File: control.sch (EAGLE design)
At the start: 63 parts

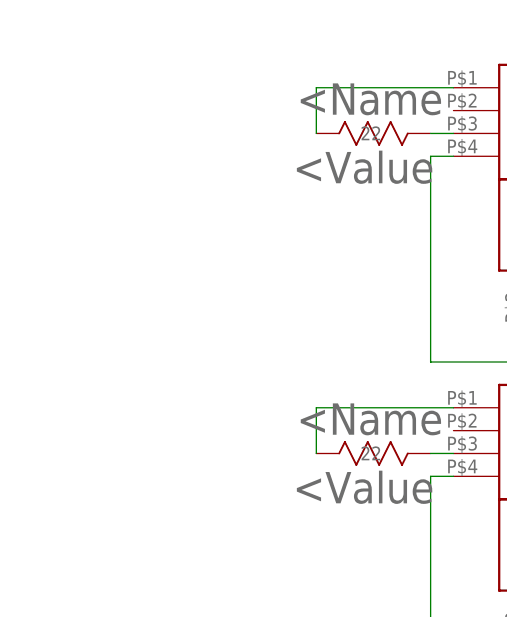
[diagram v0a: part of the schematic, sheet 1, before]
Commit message: Revert "Merge remote-tracking branch 'refs/remotes/origin/master' into new-layout"
This reverts commit d786cf153478cbc5e1d0f0cbdb23b775e7a3effd.
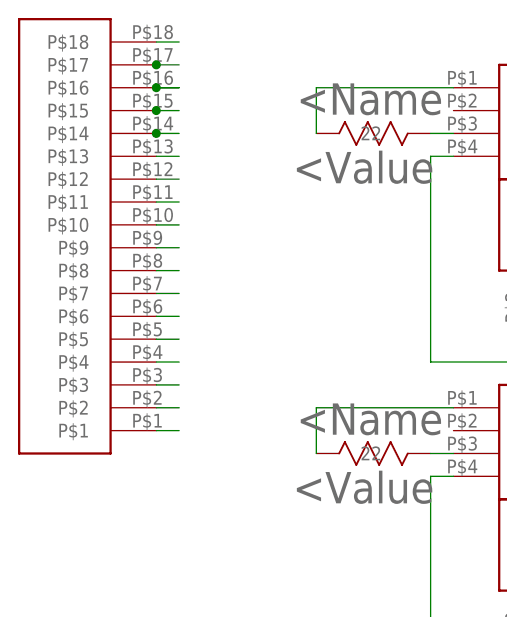
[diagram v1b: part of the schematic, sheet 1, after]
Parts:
- U$39: value MOTORCONNECTOR -> SFV18R-3STBE1HLF; device Smile_Shade:MOTORCONNECTOR -> Smile_Shade:SFV18R-3STBE1HLF
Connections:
- net LEDSTR_1: now also U$39.P$18
- net LEDSTR_10: now also U$39.P$9
- net LEDSTR_11: now also U$39.P$10
- net LEDSTR_12: now also U$39.P$7
- net LEDSTR_13: now also U$39.P$6
- net LEDSTR_14: now also U$39.P$5
- net LEDSTR_15: now also U$39.P$4
- net LEDSTR_16: now also U$39.P$3
- net LEDSTR_17: now also U$39.P$1
- net LEDSTR_18: now also U$39.P$2
- net LEDSTR_2: now also U$39.P$17
- net LEDSTR_3: now also U$39.P$16
- net LEDSTR_4: now also U$39.P$15
- net LEDSTR_5: now also U$39.P$12
- net LEDSTR_6: now also U$39.P$13
- net LEDSTR_7: now also U$39.P$14
- net LEDSTR_8: now also U$39.P$11
- net LEDSTR_9: now also U$39.P$8
- net M1A: no longer U$38.MB
- net M1B: no longer U$38.MA
- net M2A: now also U$38.MA; no longer U$39.MA
- net M2B: now also U$38.MB; no longer U$39.MB
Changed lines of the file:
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@@
 <part name="U$37" library="Smile_Shade" deviceset="PCA9685PW/Q900" device=""/>
 <part name="U$38" library="Smile_Shade" deviceset="MOTORCONNECTOR" device=""/>
-<part name="U$39" library="Smile_Shade" deviceset="MOTORCONNECTOR" device=""/>
 <part name="U$40" library="LED Driver" deviceset="NUD4011DR2G" device=""/>
 <part name="U$41" library="LED Driver" deviceset="2N7002P" device=""/>
@@
 <part name="U$43" library="LED Driver" deviceset="2N7002P" device=""/>
 <part name="R18" library="LED Driver" deviceset="RC0603FR-0710RL" device=""/>
+<part name="U$39" library="Smile_Shade" deviceset="SFV18R-3STBE1HLF" device=""/>
 </parts>
 <sheets>
@@
 <instance part="U$43" gate="G$1" x="55.88" y="-58.42"/>
 <instance part="R18" gate="A" x="30.48" y="-45.72"/>
+<instance part="U$39" gate="G$1" x="-43.18" y="60.96" rot="R90"/>
 </instances>
 <busses>
@@
 <wire x1="22.86" y1="101.6" x2="25.4" y2="101.6" width="0.1524" layer="91"/>
 </segment>
+<segment>
+<pinref part="U$39" gate="G$1" pin="P$18"/>
+<wire x1="-38.1" y1="106.68" x2="-35.56" y2="106.68" width="0.1524" layer="91"/>
+</segment>
 </net>
 <net name="N$15" class="0">
@@
 <wire x1="73.66" y1="101.6" x2="76.2" y2="101.6" width="0.1524" layer="91"/>
 </segment>
+<segment>
+<wire x1="-38.1" y1="104.14" x2="-35.56" y2="104.14" width="0.1524" layer="91"/>
+<pinref part="U$39" gate="G$1" pin="P$17"/>
+<junction x="-38.1" y="104.14"/>
+</segment>
 </net>
 <net name="N$1" class="0">
@@
 <wire x1="121.92" y1="101.6" x2="124.46" y2="101.6" width="0.1524" layer="91"/>
 </segment>
+<segment>
+<wire x1="-38.1" y1="101.6" x2="-35.56" y2="101.6" width="0.1524" layer="91"/>
+<wire x1="-38.1" y1="101.6" x2="-35.56" y2="101.6" width="0.1524" layer="91"/>
+<pinref part="U$39" gate="G$1" pin="P$16"/>
+<junction x="-38.1" y="101.6"/>
+</segment>
 </net>
 <net name="N$3" class="0">
@@
 <wire x1="172.72" y1="101.6" x2="175.26" y2="101.6" width="0.1524" layer="91"/>
 </segment>
+<segment>
+<wire x1="-38.1" y1="99.06" x2="-35.56" y2="99.06" width="0.1524" layer="91"/>
+<pinref part="U$39" gate="G$1" pin="P$15"/>
+<junction x="-38.1" y="99.06"/>
+</segment>
 </net>
 <net name="N$5" class="0">
@@
 <wire x1="22.86" y1="66.04" x2="25.4" y2="66.04" width="0.1524" layer="91"/>
 </segment>
+<segment>
+<pinref part="U$39" gate="G$1" pin="P$12"/>
+<wire x1="-38.1" y1="91.44" x2="-35.56" y2="91.44" width="0.1524" layer="91"/>
+</segment>
 </net>
 <net name="N$7" class="0">
@@
 <wire x1="73.66" y1="66.04" x2="76.2" y2="66.04" width="0.1524" layer="91"/>
 </segment>
+<segment>
+<pinref part="U$39" gate="G$1" pin="P$13"/>
+<wire x1="-38.1" y1="93.98" x2="-35.56" y2="93.98" width="0.1524" layer="91"/>
+</segment>
 </net>
 <net name="N$9" class="0">
@@
 <wire x1="121.92" y1="66.04" x2="124.46" y2="66.04" width="0.1524" layer="91"/>
 </segment>
+<segment>
+<wire x1="-38.1" y1="96.52" x2="-35.56" y2="96.52" width="0.1524" layer="91"/>
+<pinref part="U$39" gate="G$1" pin="P$14"/>
+<junction x="-38.1" y="96.52"/>
+</segment>
 </net>
 <net name="N$11" class="0">
@@
 <wire x1="172.72" y1="66.04" x2="175.26" y2="66.04" width="0.1524" layer="91"/>
 </segment>
+<segment>
+<pinref part="U$39" gate="G$1" pin="P$11"/>
+<wire x1="-38.1" y1="88.9" x2="-35.56" y2="88.9" width="0.1524" layer="91"/>
+</segment>
 </net>
 <net name="N$13" class="0">
@@
 <wire x1="22.86" y1="30.48" x2="25.4" y2="30.48" width="0.1524" layer="91"/>
 </segment>
+<segment>
+<pinref part="U$39" gate="G$1" pin="P$8"/>
+<wire x1="-38.1" y1="81.28" x2="-35.56" y2="81.28" width="0.1524" layer="91"/>
+</segment>
 </net>
 <net name="N$17" class="0">
@@
 <wire x1="73.66" y1="30.48" x2="76.2" y2="30.48" width="0.1524" layer="91"/>
 </segment>
+<segment>
+<pinref part="U$39" gate="G$1" pin="P$9"/>
+<wire x1="-38.1" y1="83.82" x2="-35.56" y2="83.82" width="0.1524" layer="91"/>
+</segment>
 </net>
 <net name="N$19" class="0">
@@
 <wire x1="121.92" y1="30.48" x2="124.46" y2="30.48" width="0.1524" layer="91"/>
 </segment>
+<segment>
+<pinref part="U$39" gate="G$1" pin="P$10"/>
+<wire x1="-38.1" y1="86.36" x2="-35.56" y2="86.36" width="0.1524" layer="91"/>
+</segment>
 </net>
 <net name="N$21" class="0">
@@
 <wire x1="172.72" y1="30.48" x2="175.26" y2="30.48" width="0.1524" layer="91"/>
 </segment>
+<segment>
+<pinref part="U$39" gate="G$1" pin="P$7"/>
+<wire x1="-38.1" y1="78.74" x2="-35.56" y2="78.74" width="0.1524" layer="91"/>
+</segment>
 </net>
 <net name="N$23" class="0">
@@
 <wire x1="22.86" y1="-5.08" x2="25.4" y2="-5.08" width="0.1524" layer="91"/>
 </segment>
+<segment>
+<pinref part="U$39" gate="G$1" pin="P$6"/>
+<wire x1="-38.1" y1="76.2" x2="-35.56" y2="76.2" width="0.1524" layer="91"/>
+</segment>
 </net>
 <net name="N$25" class="0">
@@
 <wire x1="73.66" y1="-5.08" x2="76.2" y2="-5.08" width="0.1524" layer="91"/>
 </segment>
+<segment>
+<pinref part="U$39" gate="G$1" pin="P$5"/>
+<wire x1="-38.1" y1="73.66" x2="-35.56" y2="73.66" width="0.1524" layer="91"/>
+</segment>
 </net>
 <net name="N$27" class="0">
@@
 <wire x1="121.92" y1="-5.08" x2="124.46" y2="-5.08" width="0.1524" layer="91"/>
 </segment>
+<segment>
+<pinref part="U$39" gate="G$1" pin="P$4"/>
+<wire x1="-38.1" y1="71.12" x2="-35.56" y2="71.12" width="0.1524" layer="91"/>
+</segment>
 </net>
 <net name="N$29" class="0">
@@
 <wire x1="172.72" y1="-5.08" x2="175.26" y2="-5.08" width="0.1524" layer="91"/>
 </segment>
+<segment>
+<pinref part="U$39" gate="G$1" pin="P$3"/>
+<wire x1="-38.1" y1="68.58" x2="-35.56" y2="68.58" width="0.1524" layer="91"/>
+</segment>
 </net>
 <net name="N$31" class="0">
@@
 <wire x1="22.86" y1="-40.64" x2="25.4" y2="-40.64" width="0.1524" layer="91"/>
 </segment>
+<segment>
+<pinref part="U$39" gate="G$1" pin="P$1"/>
+<wire x1="-38.1" y1="63.5" x2="-35.56" y2="63.5" width="0.1524" layer="91"/>
+</segment>
 </net>
 <net name="N$35" class="0">
@@
 <wire x1="73.66" y1="-40.64" x2="76.2" y2="-40.64" width="0.1524" layer="91"/>
 </segment>
+<segment>
+<pinref part="U$39" gate="G$1" pin="P$2"/>
+<wire x1="-38.1" y1="66.04" x2="-35.56" y2="66.04" width="0.1524" layer="91"/>
+</segment>
 </net>
 <net name="N$37" class="0">
@@
 <instance part="C2" gate="A" x="104.14" y="68.58"/>
 <instance part="U$37" gate="G$1" x="213.36" y="43.18"/>
-<instance part="U$38" gate="G$1" x="76.2" y="25.4" rot="R180"/>
-<instance part="U$39" gate="G$1" x="218.44" y="27.94"/>
+<instance part="U$38" gate="G$1" x="218.44" y="27.94"/>
 </instances>
 <busses>
@@
 <segment>
 <wire x1="83.82" y1="30.48" x2="83.82" y2="27.94" width="0.1524" layer="91"/>
-<pinref part="U$38" gate="G$1" pin="MB"/>
-<wire x1="83.82" y1="27.94" x2="81.28" y2="27.94" width="0.1524" layer="91"/>
 <pinref part="U$2" gate="A" pin="1Y"/>
 <wire x1="83.82" y1="30.48" x2="88.9" y2="30.48" width="0.1524" layer="91"/>
@@
 <net name="M2B" class="0">
 <segment>
-<pinref part="U$39" gate="G$1" pin="MB"/>
 <wire x1="213.36" y1="25.4" x2="213.36" y2="22.86" width="0.1524" layer="91"/>
 <pinref part="U$2" gate="A" pin="3Y"/>
 <wire x1="205.74" y1="22.86" x2="213.36" y2="22.86" width="0.1524" layer="91"/>
+<pinref part="U$38" gate="G$1" pin="MB"/>
 </segment>
 </net>
@@
 <wire x1="88.9" y1="22.86" x2="83.82" y2="22.86" width="0.1524" layer="91"/>
 <wire x1="83.82" y1="22.86" x2="83.82" y2="25.4" width="0.1524" layer="91"/>
-<pinref part="U$38" gate="G$1" pin="MA"/>
-<wire x1="83.82" y1="25.4" x2="81.28" y2="25.4" width="0.1524" layer="91"/>
 </segment>
 </net>
@@
 <segment>
 <pinref part="U$2" gate="A" pin="4Y"/>
-<pinref part="U$39" gate="G$1" pin="MA"/>
 <wire x1="205.74" y1="30.48" x2="213.36" y2="30.48" width="0.1524" layer="91"/>
 <wire x1="213.36" y1="30.48" x2="213.36" y2="27.94" width="0.1524" layer="91"/>
-</segment>
-</net>
+<pinref part="U$38" gate="G$1" pin="MA"/>
+</segment>
+</net>
